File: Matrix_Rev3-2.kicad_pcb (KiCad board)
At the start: 2 copper layers, 34 parts, among them SW1 DPST, SW10 DPST, SW11 DPST, SW12 DPST, SW13 DPST, SW14 DPST, SW15 DPST, SW16 DPST, SW2 DPST, SW3 DPST, SW4 DPST, SW5 DPST, SW6 DPST, SW7 DPST, SW8 DPST, SW9 DPST

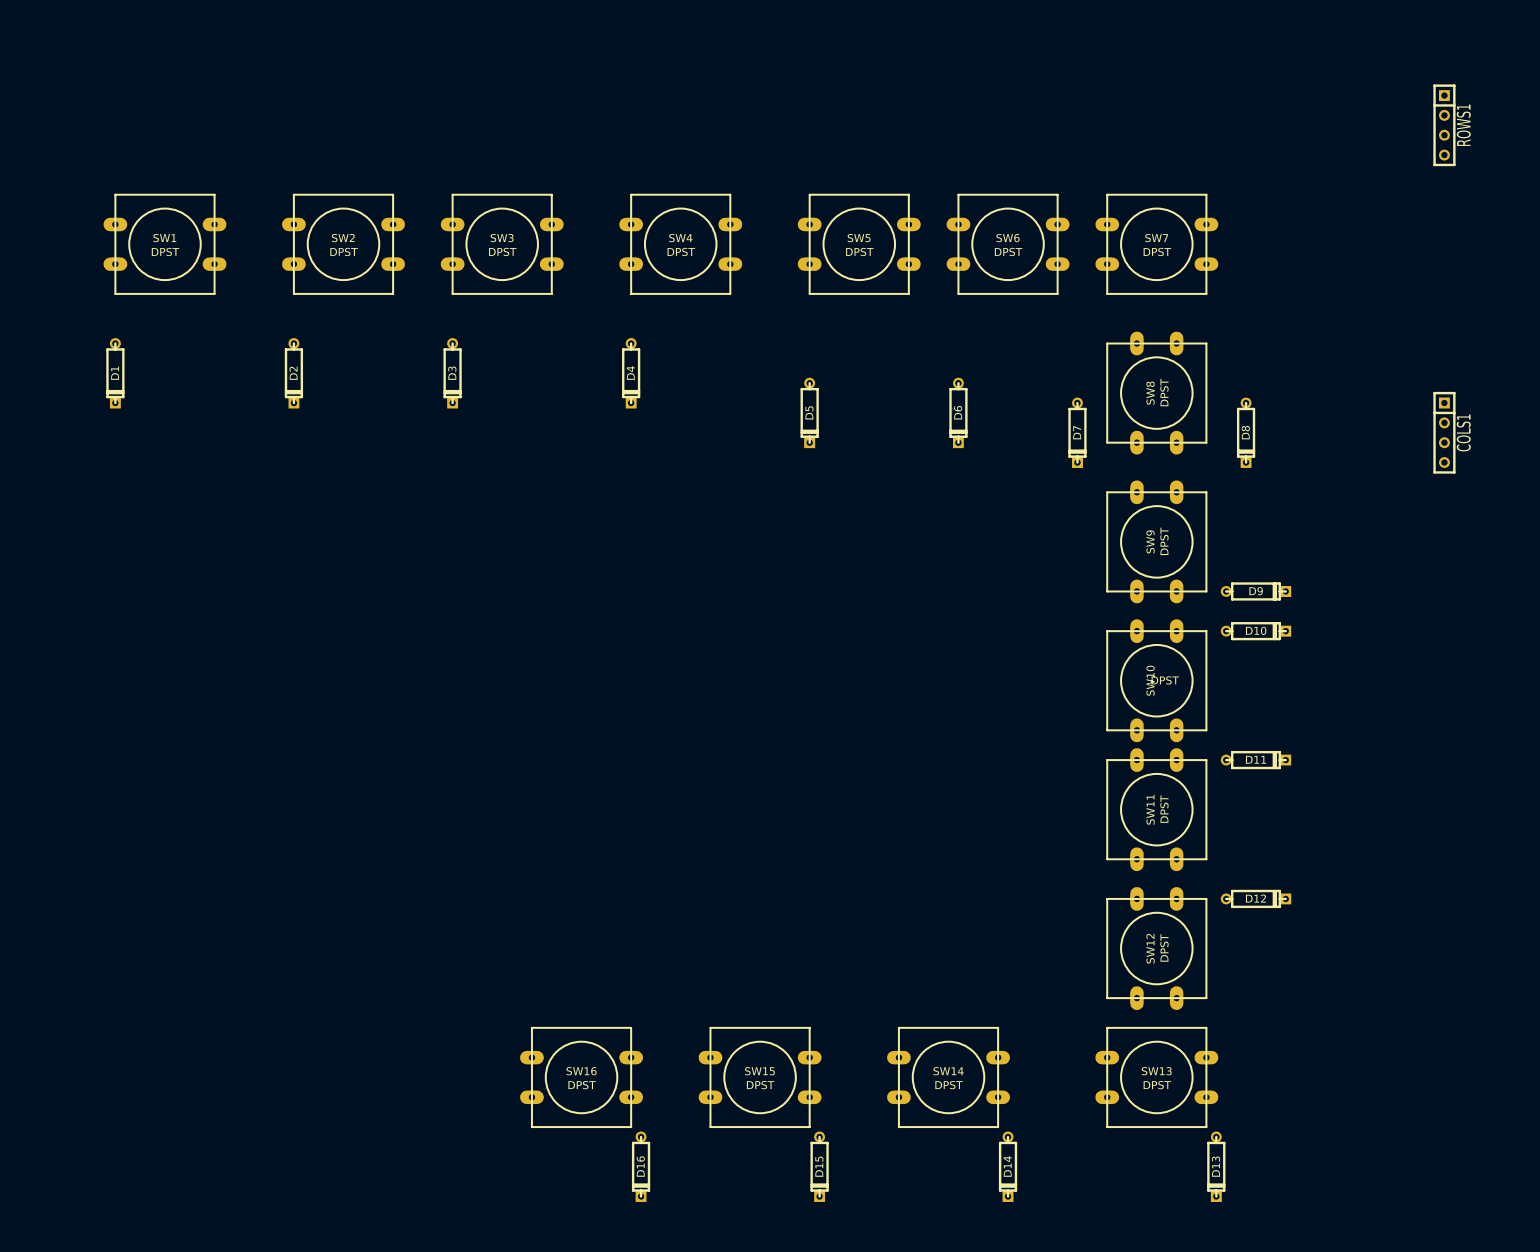
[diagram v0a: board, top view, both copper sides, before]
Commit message: Started track tracing
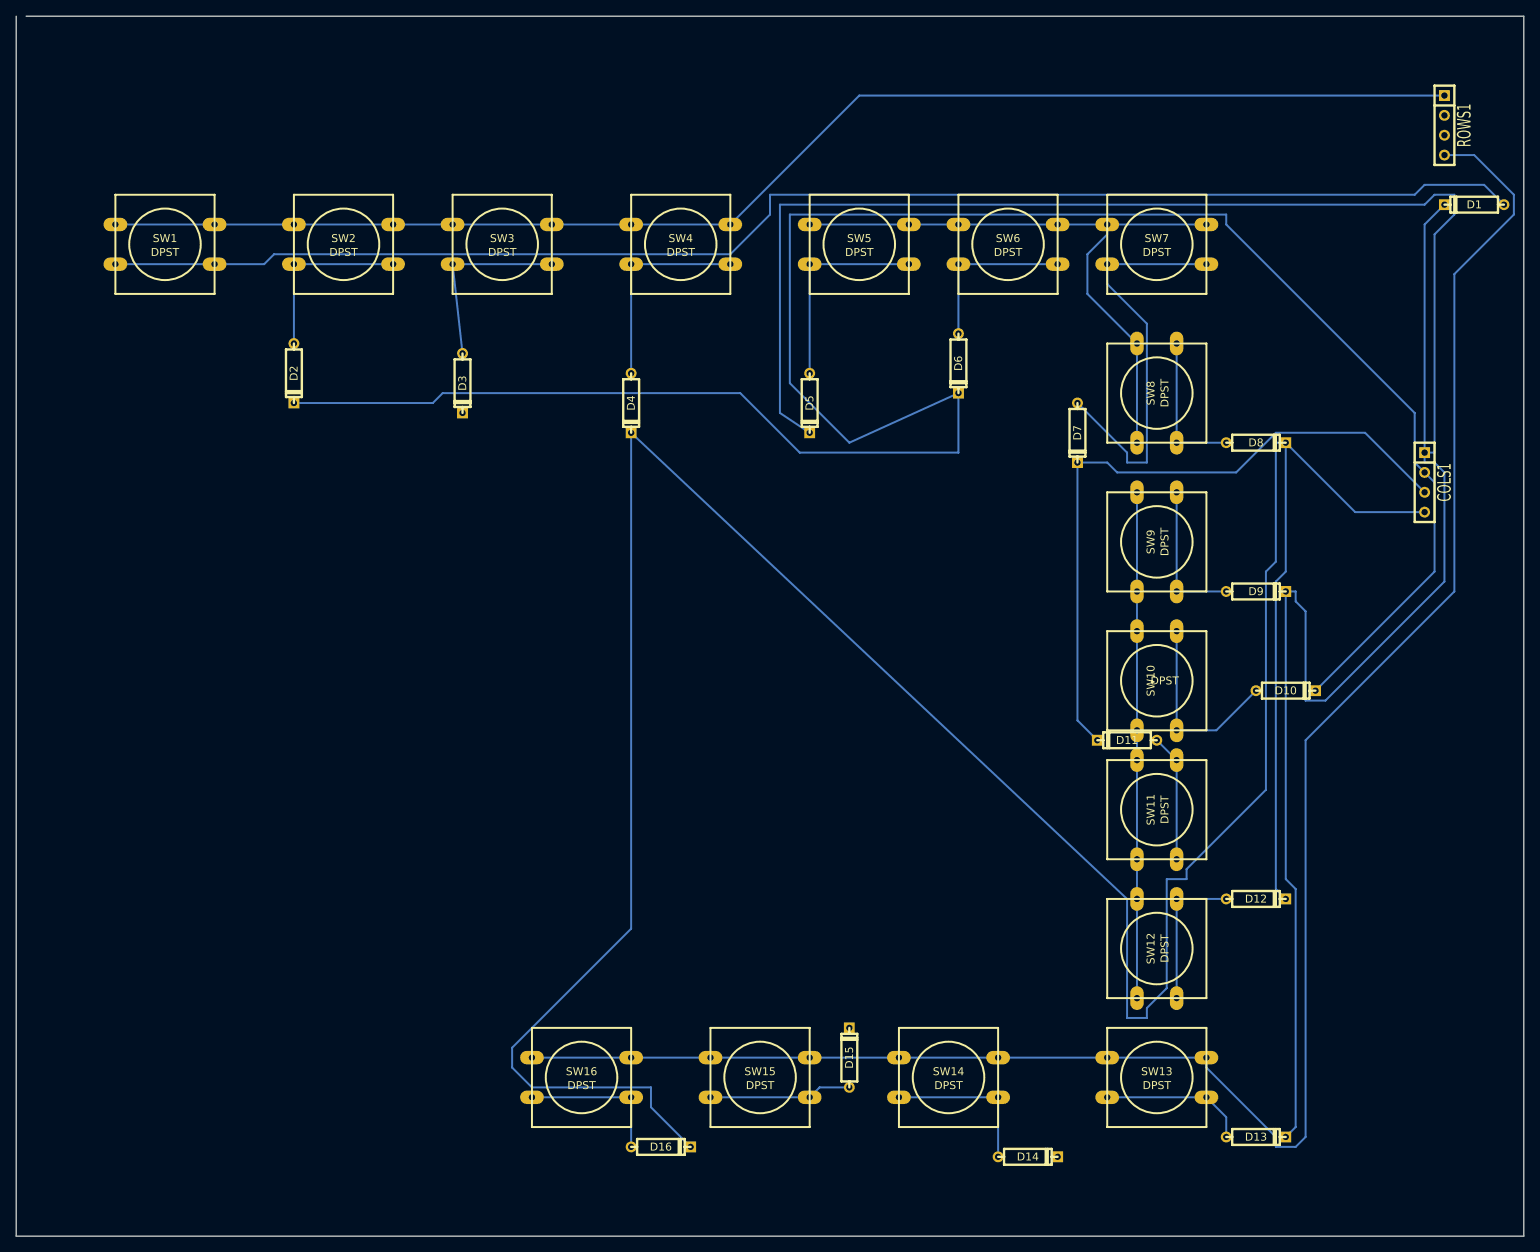
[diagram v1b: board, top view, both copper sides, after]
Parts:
- moved D1 175.3 mm to (348.0, 106.7), turned to 180 degrees
- moved D11 16.7 mm to (303.5, 175.3), turned to 180 degrees
- moved D15 14.5 mm to (268.0, 215.9), turned to 90 degrees
- moved D10 8.52 mm to (323.9, 168.9)
- moved COLS1 6.84 mm to (341.6, 142.2)
- moved D13 6.35 mm to (320.0, 226.1), turned to 0 degrees
- moved D6 6.35 mm to (281.9, 127.0)
- moved D4 3.81 mm to (240.0, 132.1)
- moved D16 3.59 mm to (243.8, 227.3), turned to 0 degrees
- moved D14 2.84 mm to (290.8, 228.6), turned to 0 degrees
- moved D8 1.80 mm to (320.0, 137.2), turned to 0 degrees
- moved D3 1.80 mm to (218.4, 129.5)
- moved D5 1.27 mm to (262.9, 132.1)
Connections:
- D10 pad 2: /c3 -> /c2
- D12 pad 2: /c3 -> /c4
- D13 pad 2: /c4 -> /c1
- D14 pad 2: /c4 -> /c2
- D15 pad 2: /c4 -> /c3
- D2 pad 2: /c1 -> /c2
- D3 pad 2: /c1 -> /c3
- D4 pad 2: /c1 -> /c4
- D5 pad 2: /c2 -> /c1
- D7 pad 2: /c2 -> /c3
- D8 pad 2: /c2 -> /c4
- D9 pad 2: /c3 -> /c1
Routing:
- net /c4: track 0.00 -> 385.3 mm
- net /c1: track 0.00 -> 315.3 mm
- net /c2: track 0.00 -> 278.3 mm
- net /a4: track 0.00 -> 248.5 mm
- net N-0000014: track 0.00 -> 184.5 mm
- net /a1: track 0.00 -> 177.0 mm
- net /c3: track 0.00 -> 86.8 mm
- net /a2: track 0.00 -> 82.4 mm
- net /a3: track 0.00 -> 64.8 mm
- net N-0000022: track 0.00 -> 53.0 mm
- net N-0000024: track 0.00 -> 26.7 mm
- net N-0000019: track 0.00 -> 26.7 mm
- net N-0000010: track 0.00 -> 25.0 mm
- net N-0000018: track 0.00 -> 24.2 mm
- net N-0000017: track 0.00 -> 22.9 mm
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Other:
- board outline added: 193 x 156.2 mm
